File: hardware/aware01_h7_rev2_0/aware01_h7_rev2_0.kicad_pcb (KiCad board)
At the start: 4 copper layers, 46 x 110 mm, 157 parts, among them IC1 587-2054-127F, IC2 587-2054-127F, IC3 587-2054-127F, IC4 587-2054-127F, IC5 TLV320AIC3204IRHBR, J1 Conn_02x07_Odd_Even, J10 GATE4_IN, J11 CV2_IN, J12 CV3_IN, J13 V/OCT_IN, J14 CV1_IN, J2 Conn_02x05_Odd_Even, J3 InL, J4 InR, J5 OutL, J6 OutR, J7 GATE1_IN, J8 GATE2_IN, J9 GATE3_IN, Q1 MMBT3904, Q2 MMBT3904, Q3 MMBT3904, Q4 MMBT3904, SW1 SW_Push, SW2 SW_Push, SW3 PTS815, U1 LMR50410Y5FQDBVRQ1, U10 NE5532DRG4, U11 NE5532DRG4, U12 OPA2322AIDR, U13 OPA2322AIDR, U2 LM1117MP-3.3, U3 74AHCT1G14DBVRG4, U4 STM32H7A3RITx, U5 LM4040DIM3X-10, U6 10k, U7 10k, U8 10k, U9 10k, Y1 WE-XTAL 24.0MHz 50ppm

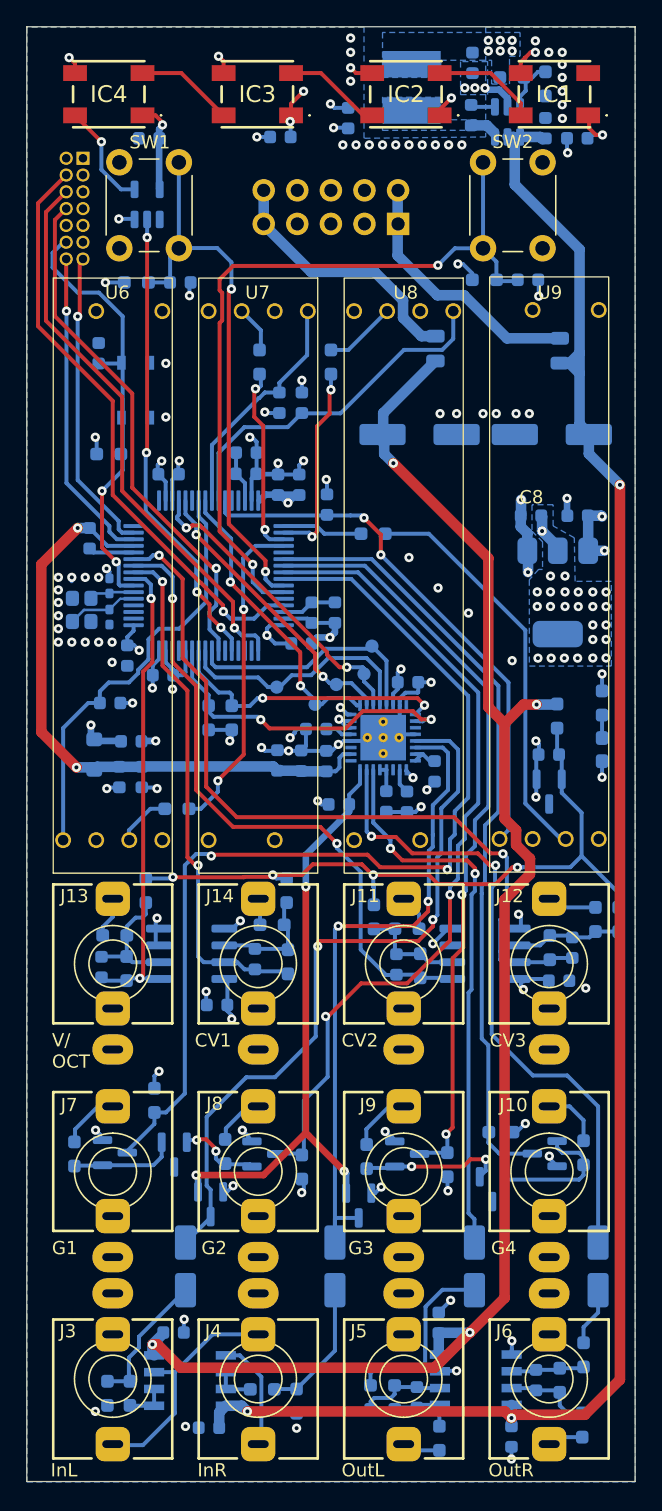
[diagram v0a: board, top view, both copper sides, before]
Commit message: hw: improve layout
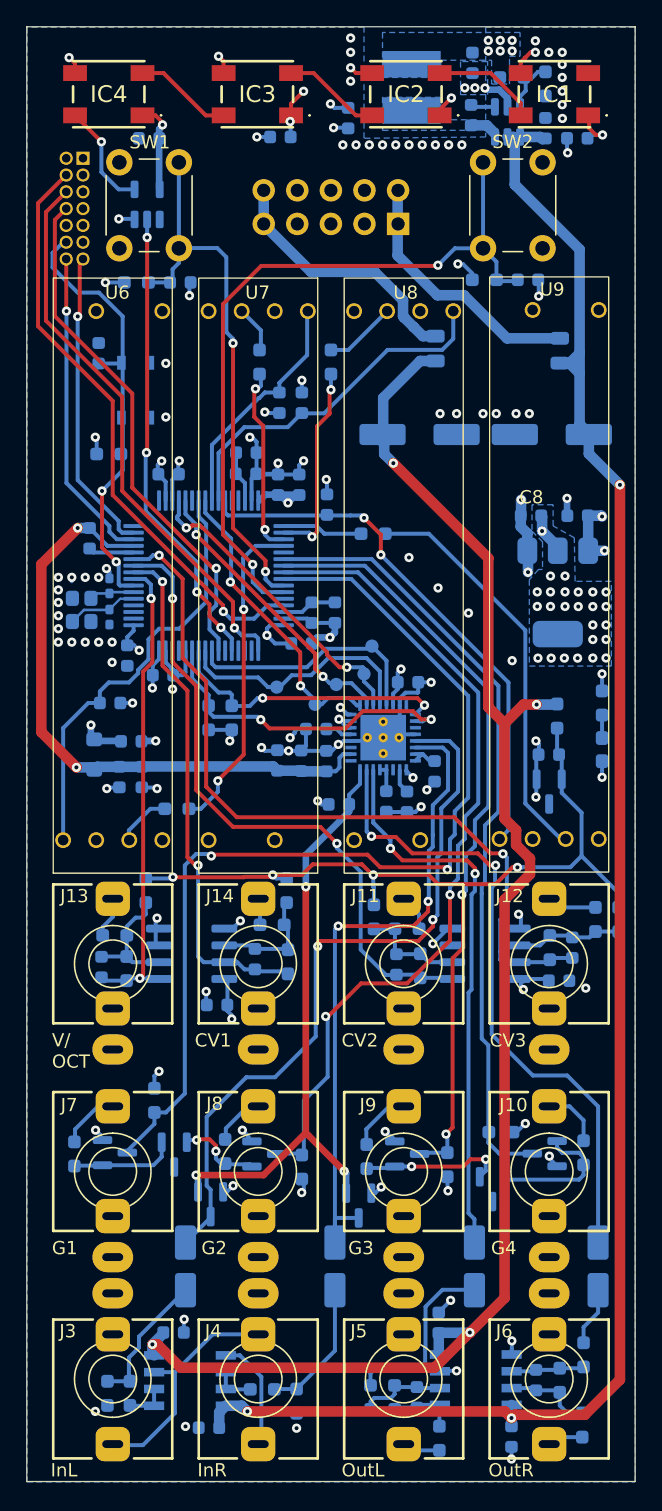
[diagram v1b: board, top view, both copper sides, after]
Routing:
- net /BUTTON2_IN: track 58.9 -> 57.2 mm
- net -12V: track 117.8 -> 118.5 mm
